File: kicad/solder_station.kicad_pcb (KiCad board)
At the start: 2 copper layers, 77.8 x 66.5 mm, 42 parts, among them IC1 ATMEGA328-P, P1 CONN_01X05, P2 CONN_01X02, P3 Standby, P4 UART, Q1 2N7000, Q2 IRF4905, T1 Measurement_Point_Round-TH_Big, U1 LM2596_module, U2 AD8572, U3 EC11, Y1 16MHz

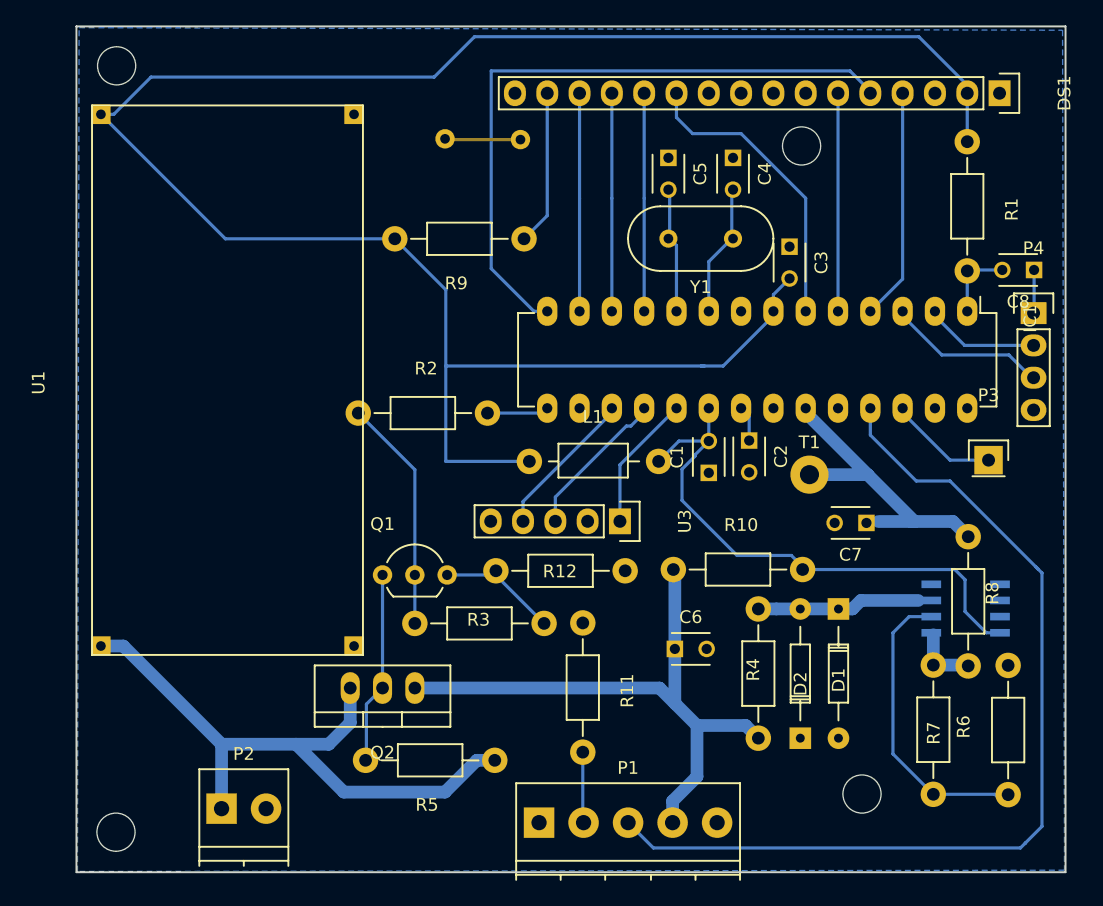
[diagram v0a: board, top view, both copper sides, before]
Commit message: [Kicad] Update schematics. Using ad8551.
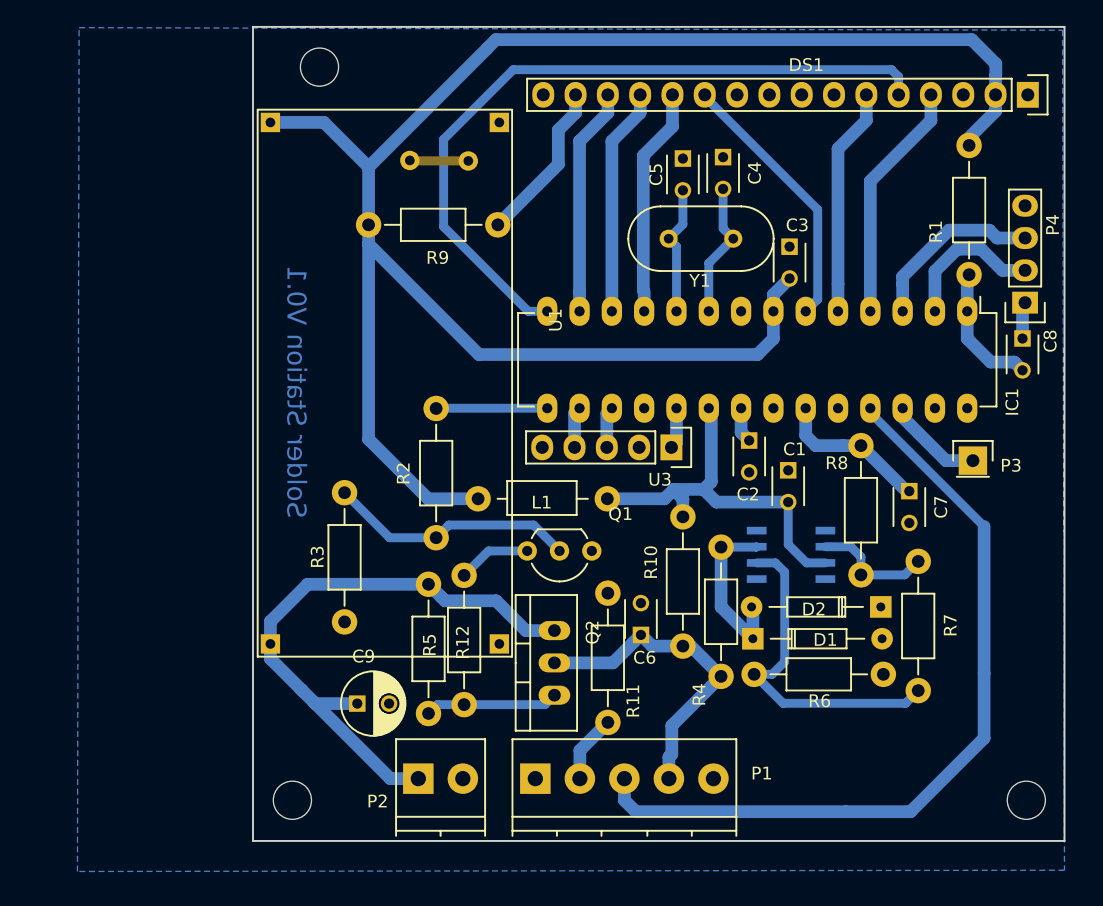
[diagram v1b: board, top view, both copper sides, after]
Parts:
- removed Hole4: MountingHole_3mm, Mounting_Holes:MountingHole_3mm
- removed T1: Measurement_Point_Round-TH_Big, Measurement_Points:Measurement_Point_Round-TH_Big
- added C9: CP, Capacitors_ThroughHole:C_Radial_D5_L11_P2.5, F.Cu at (112.7, 117.2)
- R10: value 1MΩ -> 300kΩ
- R12, R5: value 10kΩ -> 1kΩ
- R6: value 100Ω -> 1kΩ
- R7: value 50kΩ -> 100kΩ
- moved Q1 16.6 mm to (131.1, 105.2), turned to 180 degrees
- moved Hole3 16.0 mm to (109.7, 67.2)
- moved P2 15.6 mm to (117.5, 123.1)
- moved R6 15.5 mm to (149.0, 114.9), turned to 0 degrees
- moved U2 14.4 mm to (146.8, 105.5)
- moved Hole2 14.1 mm to (107.6, 124.8)
- moved U1 14.1 mm to (105.9, 112.5)
- moved Q2 13.7 mm to (128.2, 114.0), turned to 90 degrees
- moved Hole1 12.9 mm to (165.3, 124.8)
- moved D2 12.1 mm to (153.9, 109.6), turned to 180 degrees
- moved R3 11.8 mm to (111.7, 105.7), turned to 270 degrees
- moved R8 11.1 mm to (152.3, 102.0)
- moved R12 9.33 mm to (121.1, 112.2), turned to 90 degrees
- moved R5 8.76 mm to (118.3, 112.9), turned to 270 degrees
- moved R7 8.24 mm to (156.8, 111.1)
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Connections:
- DS1 pad 10: Net-(DS1-Pad10) -> (no net)
- DS1 pad 7: Net-(DS1-Pad7) -> (no net)
- DS1 pad 8: Net-(DS1-Pad8) -> (no net)
- DS1 pad 9: Net-(DS1-Pad9) -> (no net)
- IC1 pad 16: Net-(IC1-Pad16) -> /Button_push
- IC1 pad 17: /Button_push -> /Rotary_B
- IC1 pad 18: /Rotary_B -> (no net)
- IC1 pad 24: Net-(IC1-Pad24) -> (no net)
- IC1 pad 27: Net-(IC1-Pad27) -> (no net)
- IC1 pad 28: Net-(IC1-Pad28) -> (no net)
- Q1 pad 1: Net-(Q1-Pad1) -> GND
- Q2 pad 1: /Heater+ -> Net-(Q2-Pad1)
- Q2 pad 2: Net-(Q1-Pad1) -> /Heater+
- R12 pad 1: Net-(Q1-Pad3) -> Net-(Q2-Pad1)
- R12 pad 2: GND -> Net-(Q1-Pad3)
- R3 pad 2: Net-(Q1-Pad3) -> GND
- R5 pad 2: Net-(Q1-Pad1) -> Net-(Q2-Pad1)
- U2 pad 1: Net-(R7-Pad1) -> (no net)
- U2 pad 6: (no net) -> Net-(R7-Pad1)
- U2 pad 7: (no net) -> AVcc
- U2 pad 8: AVcc -> (no net)
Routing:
- net /Heater+: track 48.5 -> 25.1 mm
- net +5V: track 161.0 -> 143.6 mm
- net Net-(Q1-Pad1): track 15.1 -> 0.00 mm
- net /Temp_sense: track 26.0 -> 12.1 mm
- net AVcc: track 44.4 -> 30.7 mm
- net /Button_connected: track 74.8 -> 62.4 mm
- net Net-(Q2-Pad1): track 0.00 -> 10.5 mm
- net /Rotary_B: track 12.0 -> 3.24 mm
- net /Button_push: track 11.8 -> 3.24 mm
- net /Rotary_A: track 11.6 -> 3.24 mm
- net /LCD_RW: track 52.0 -> 58.1 mm
- net Net-(R7-Pad1): track 5.47 -> 9.48 mm
- net Net-(Q1-Pad3): track 9.67 -> 5.76 mm
- net /Heater_PWM: track 4.86 -> 8.72 mm
- net Net-(R6-Pad1): track 22.9 -> 26.6 mm
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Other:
- board size 77.8 x 66.5 mm -> 63.8 x 64 mm
- net class Default: clearance 0.2 -> 0.5; trace_width 0.25 -> 0.7
- net class Power: clearance 0.2 -> 0.5
- rule trace_clearance: 0.2 -> 0.5
- rule trace_min: 0.2 -> 0.7
- board text added: "Solder Station V0.1"
